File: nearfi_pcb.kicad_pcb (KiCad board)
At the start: 4 copper layers, 45.6 x 45.6 mm, 50 parts, among them J1 PWR_CNN, J2 PROG_CNN, Q1 MMBT3904, SW1 SRST_BTN, U2 TLV1117-33, U3 AT24CS02-STUM, U4 TPL5010, U5 ESP32-S3-MINI-1

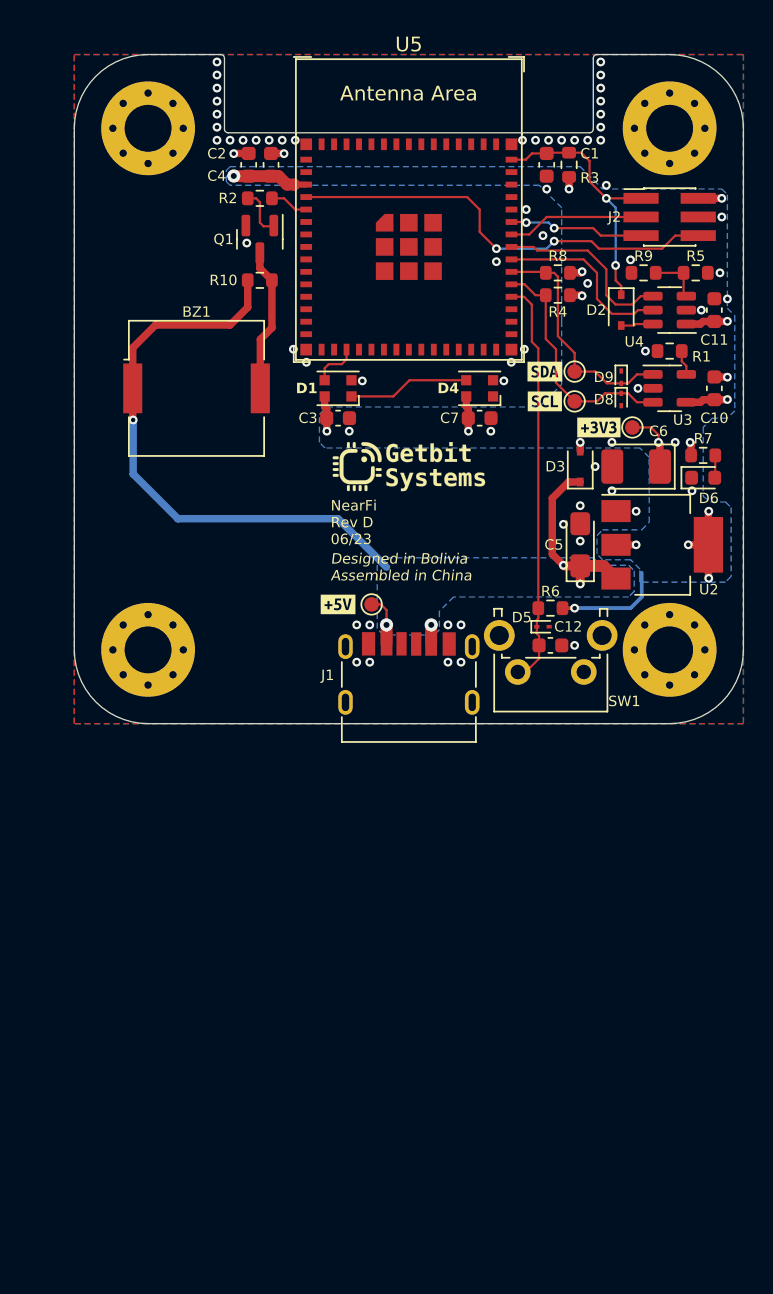
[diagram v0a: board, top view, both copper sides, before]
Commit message: updated schematic and layout
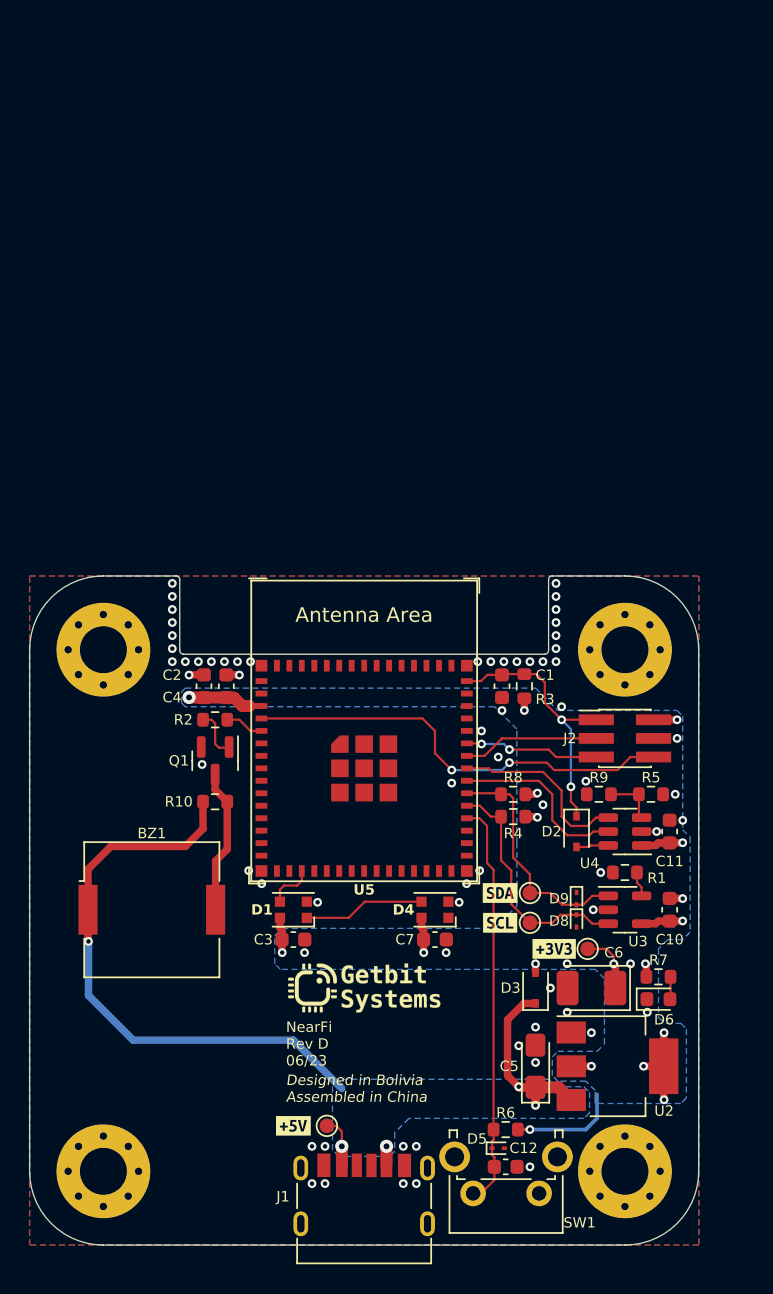
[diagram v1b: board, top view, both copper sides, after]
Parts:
- moved C6 35.7 mm to (161.8, 103.9)
- moved D3 35.7 mm to (158.0, 103.9)
- moved D6 35.7 mm to (166.4, 104.6)
- moved G*** 35.7 mm to (146.3, 103.9)
- moved R6 35.7 mm to (156.0, 113.5)
- moved R7 35.7 mm to (166.4, 103.1)
- moved BZ1 35.7 mm to (131.8, 98.5)
- moved C1 35.7 mm to (155.7, 83.3)
- moved C10 35.7 mm to (167.1, 98.5)
- moved C2 35.7 mm to (135.4, 83.3)
- moved C4 35.7 mm to (136.9, 83.3)
- moved D1 35.7 mm to (141.5, 98.5)
- moved D4 35.7 mm to (151.1, 98.5)
- moved D8 35.7 mm to (160.8, 99.3)
- moved D9 35.7 mm to (160.8, 97.8)
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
